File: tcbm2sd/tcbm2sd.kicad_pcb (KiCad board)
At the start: 2 copper layers, 56 x 91 mm, 27 parts, among them J1 TCBM, J2 JTAG, J4 AMS1117, J5 SD CARD, J7 ALT_A6_A7, SW1 BUT_PREV, SW2 BUT_NEXT, U1 XC9572XL-VQ64, U2 Arduino Pro Mini, U3 AMS1117-3.3, U4 27C512

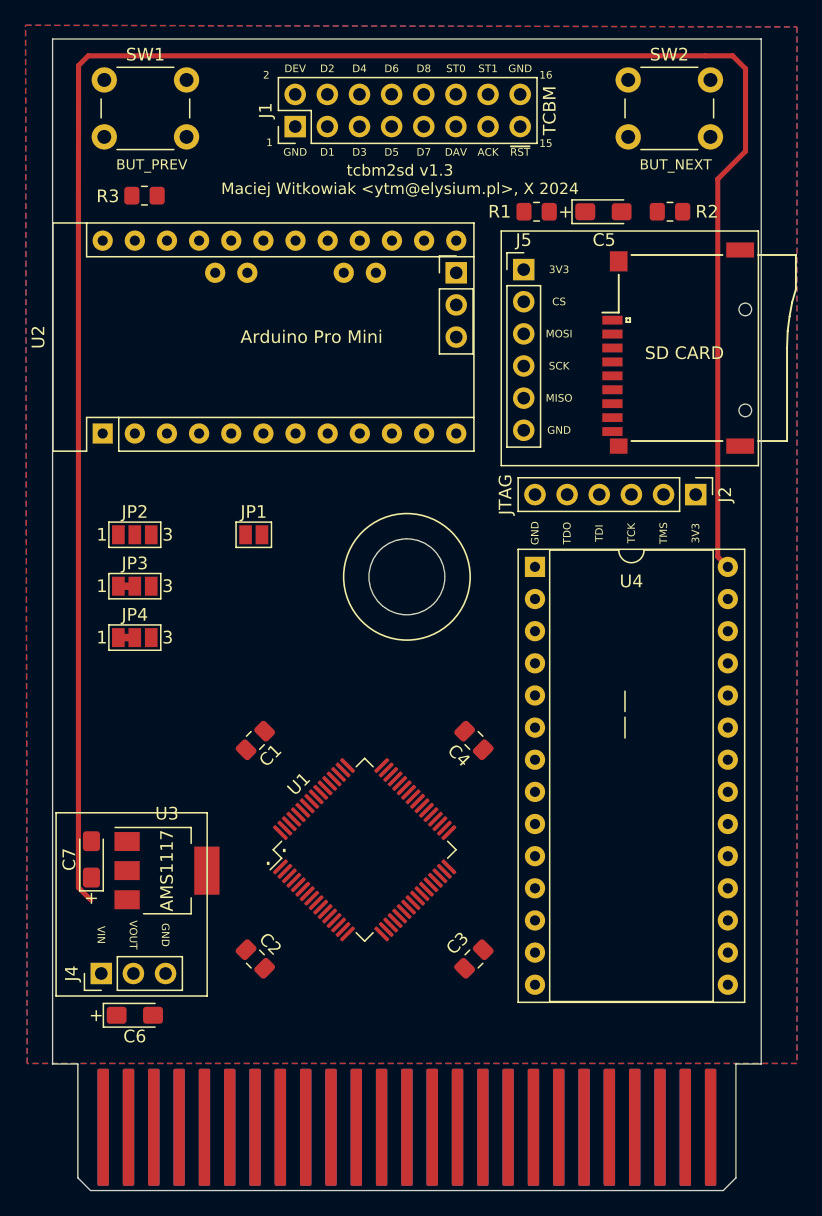
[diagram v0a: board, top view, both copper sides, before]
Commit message: updated routing
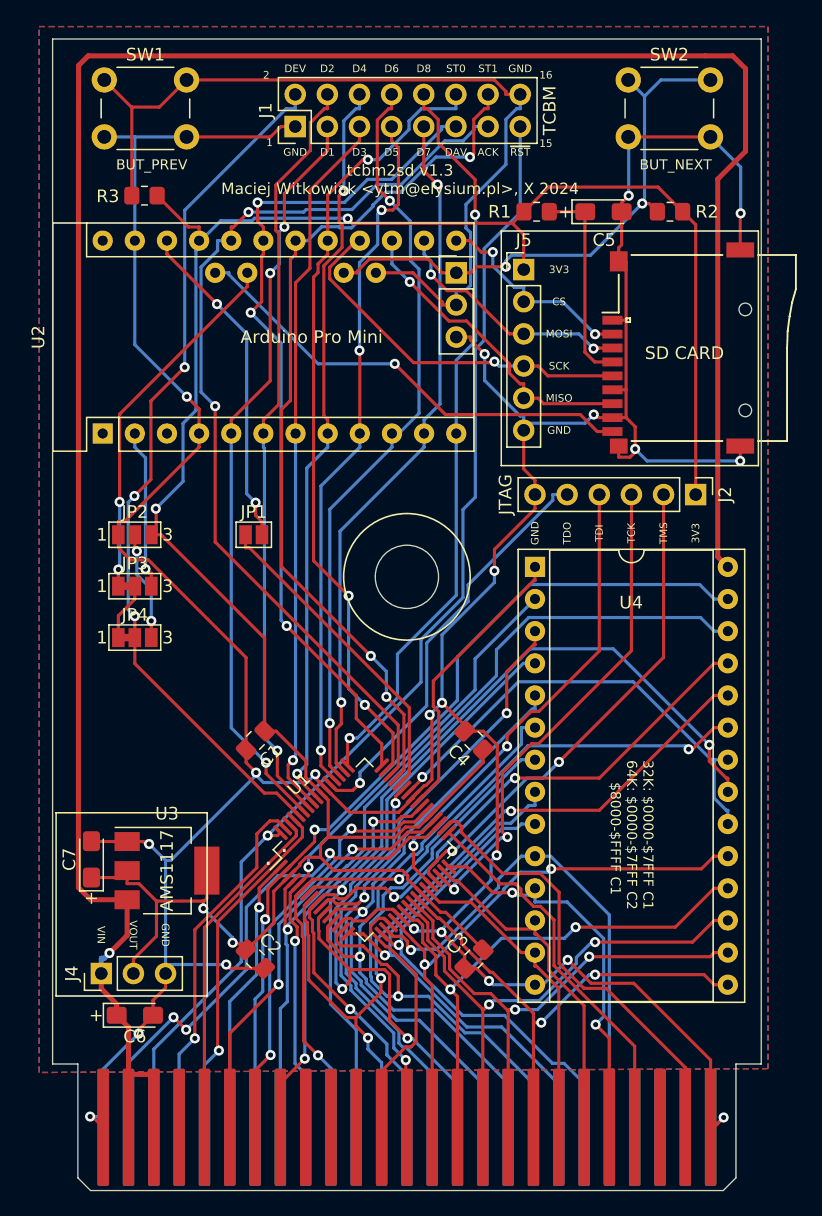
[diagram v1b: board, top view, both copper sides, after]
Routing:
- net GND: track 0.00 -> 313.4 mm, vias 0 -> 22
- net +3V3: track 0.00 -> 196.3 mm, vias 0 -> 4
- net /~{RESET}: track 0.00 -> 92.2 mm, vias 0 -> 1
- net /ACK: track 0.00 -> 75.3 mm, vias 0 -> 2
- net /A10: track 0.00 -> 70.0 mm, vias 0 -> 2
- net /STATUS1: track 0.00 -> 69.7 mm, vias 0 -> 3
- net /ALT_A6: track 0.00 -> 69.4 mm
- net /A13: track 0.00 -> 69.0 mm, vias 0 -> 1
- net /DEV: track 0.00 -> 68.9 mm, vias 0 -> 3
- net /A14: track 0.00 -> 68.6 mm, vias 0 -> 2
- net /DAV: track 0.00 -> 67.7 mm, vias 0 -> 3
- net /A9: track 0.00 -> 64.2 mm, vias 0 -> 3
- net /STATUS0: track 0.00 -> 63.2 mm, vias 0 -> 3
- net /DIO2: track 0.00 -> 60.1 mm, vias 0 -> 1
- net /A11: track 0.00 -> 59.5 mm, vias 0 -> 3
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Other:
- board text added: "32K: $0000-$7FFF C1 64K: $0000-$7FFF C2 $8000-$FFFF C1"
